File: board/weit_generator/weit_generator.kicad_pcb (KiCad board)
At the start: 2 copper layers, 56.3 x 59.7 mm, 61 parts, among them J1 Zasilanie, J2 PROG, J3 Wyjście, Q1 BC547, U1 AVR32DA28x-xSO, U2 MCP6004, U3 LM4041L, X1 SG-5032CAN

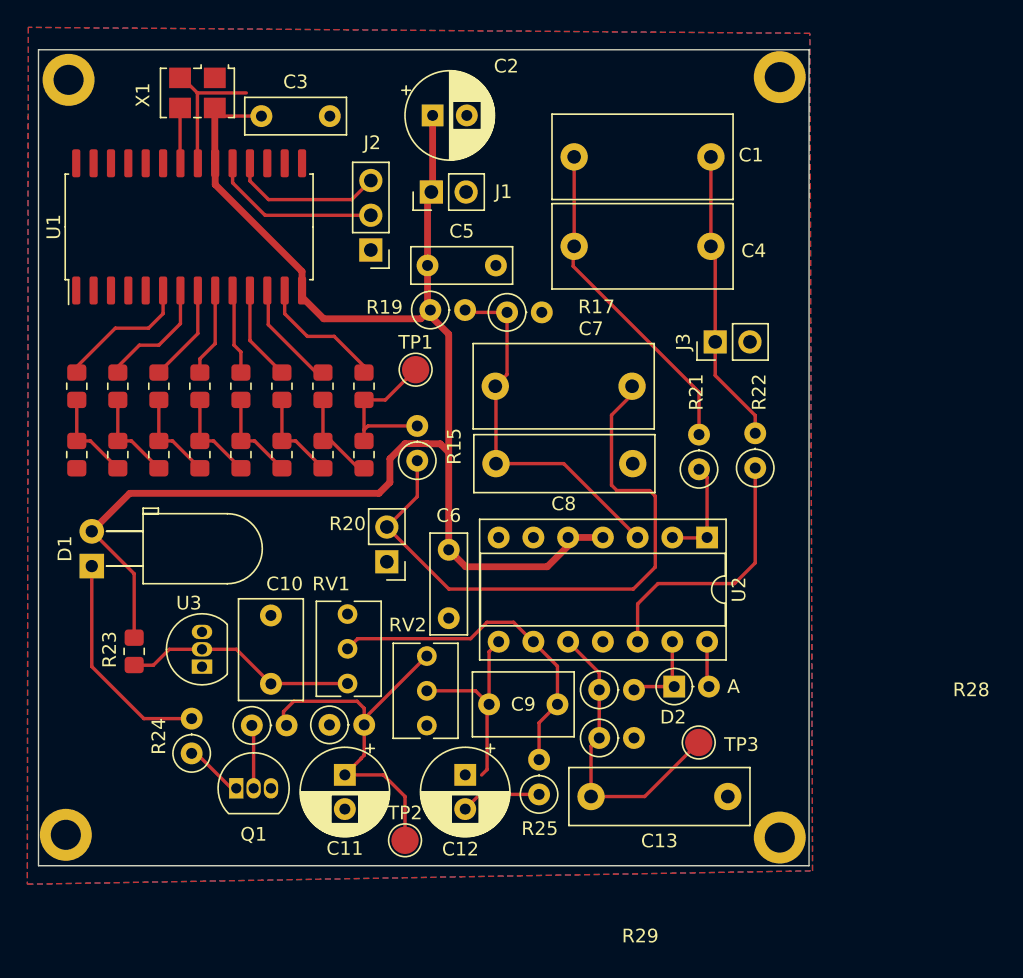
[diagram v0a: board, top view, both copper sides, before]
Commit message: potężny polski assembler
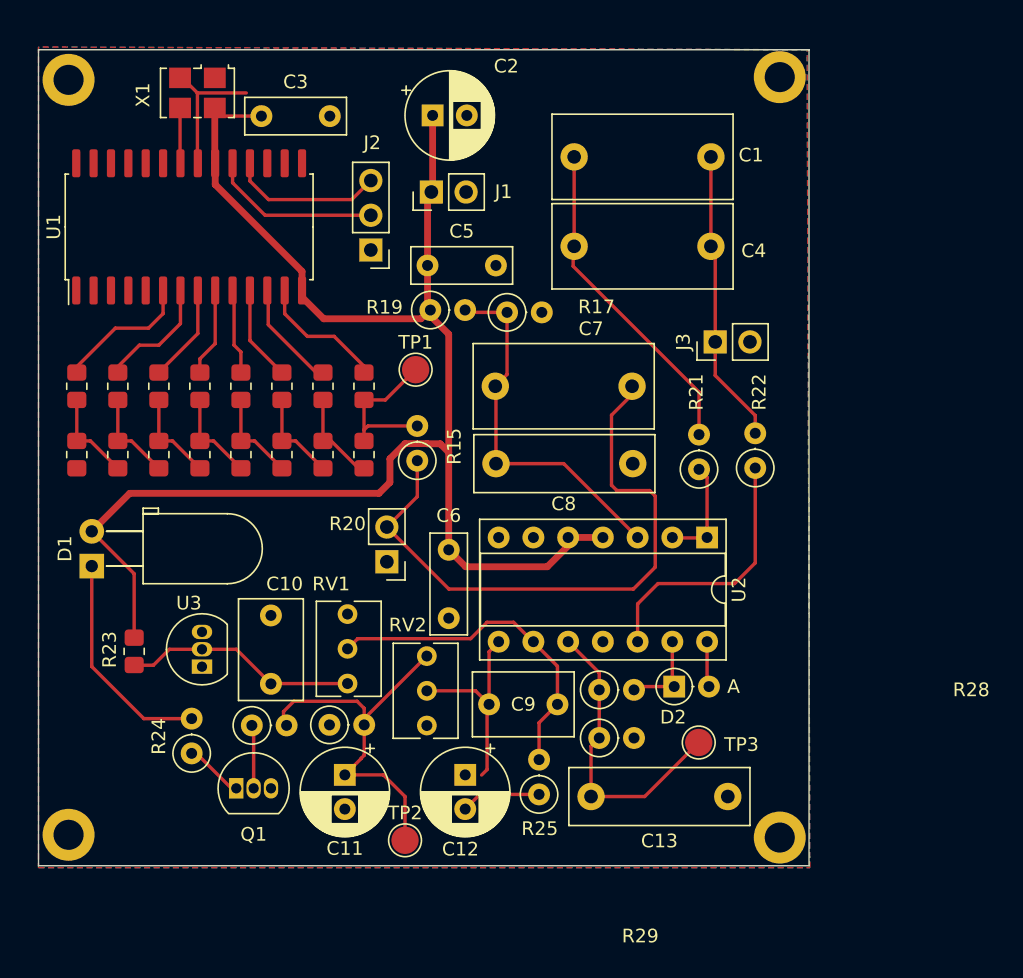
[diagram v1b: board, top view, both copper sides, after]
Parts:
- moved REF** 0.20 mm to (101.2, 133.6)
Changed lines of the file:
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@@
       (sketchpadsonfab false)
       (subtractmaskfromsilk false)
-      (outputformat 1)
+      (outputformat 4)
       (mirror false)
       (drillshape 0)
       (scaleselection 1)
-      (outputdirectory "grb")
+      (outputdirectory "../../../../")
     )
   )
@@
   )
   (footprint "MountingHole:MountingHole_2.2mm_M2_DIN965_Pad" (layer "F.Cu")
-    (at 101 133.6)
+    (at 101.2 133.6)
     (descr "Mounting Hole 2.2mm, M2, DIN965")
     (tags "mounting hole 2.2mm m2 din965")
@@
     (polygon
       (pts
-        (xy 155.595542 136.230795)
-        (xy 155.4 75)
-        (xy 98.255542 74.560795)
-        (xy 98.185542 137.210795)
+        (xy 155.4 136)
+        (xy 155.2 76.2)
+        (xy 99 76)
+        (xy 99 136)
       )
     )
